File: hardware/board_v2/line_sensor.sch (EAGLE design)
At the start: 64 parts, among them J1 XF2L-0535-1, Q1 BSS123

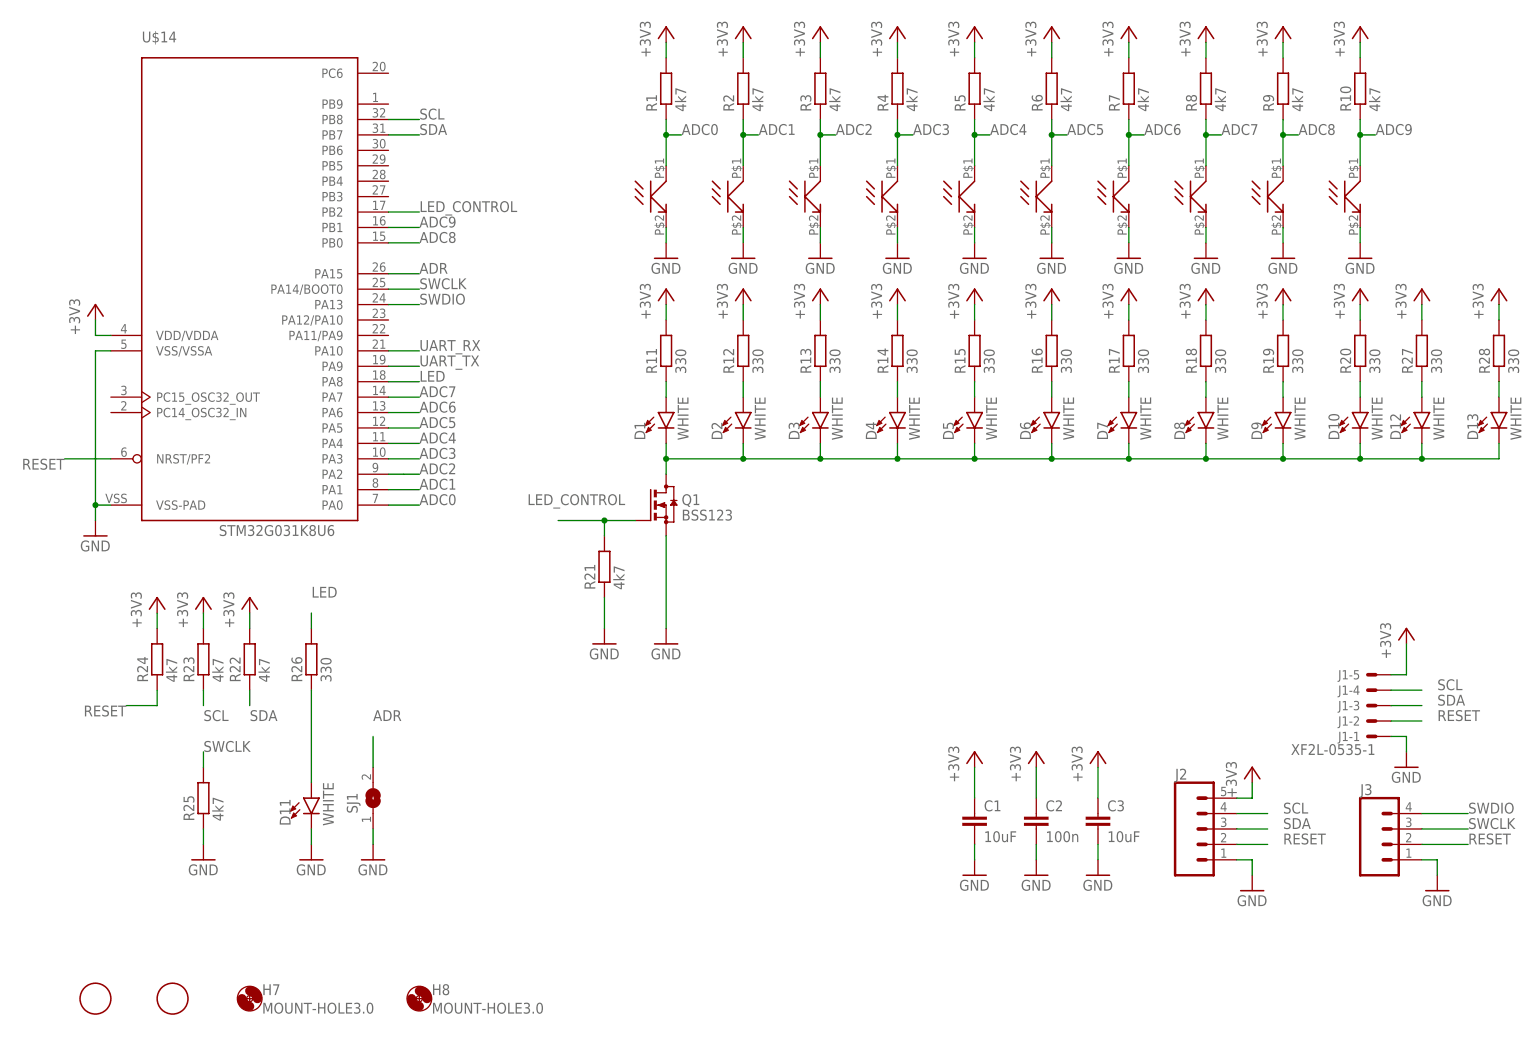
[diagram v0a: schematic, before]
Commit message: updated v2 firmware
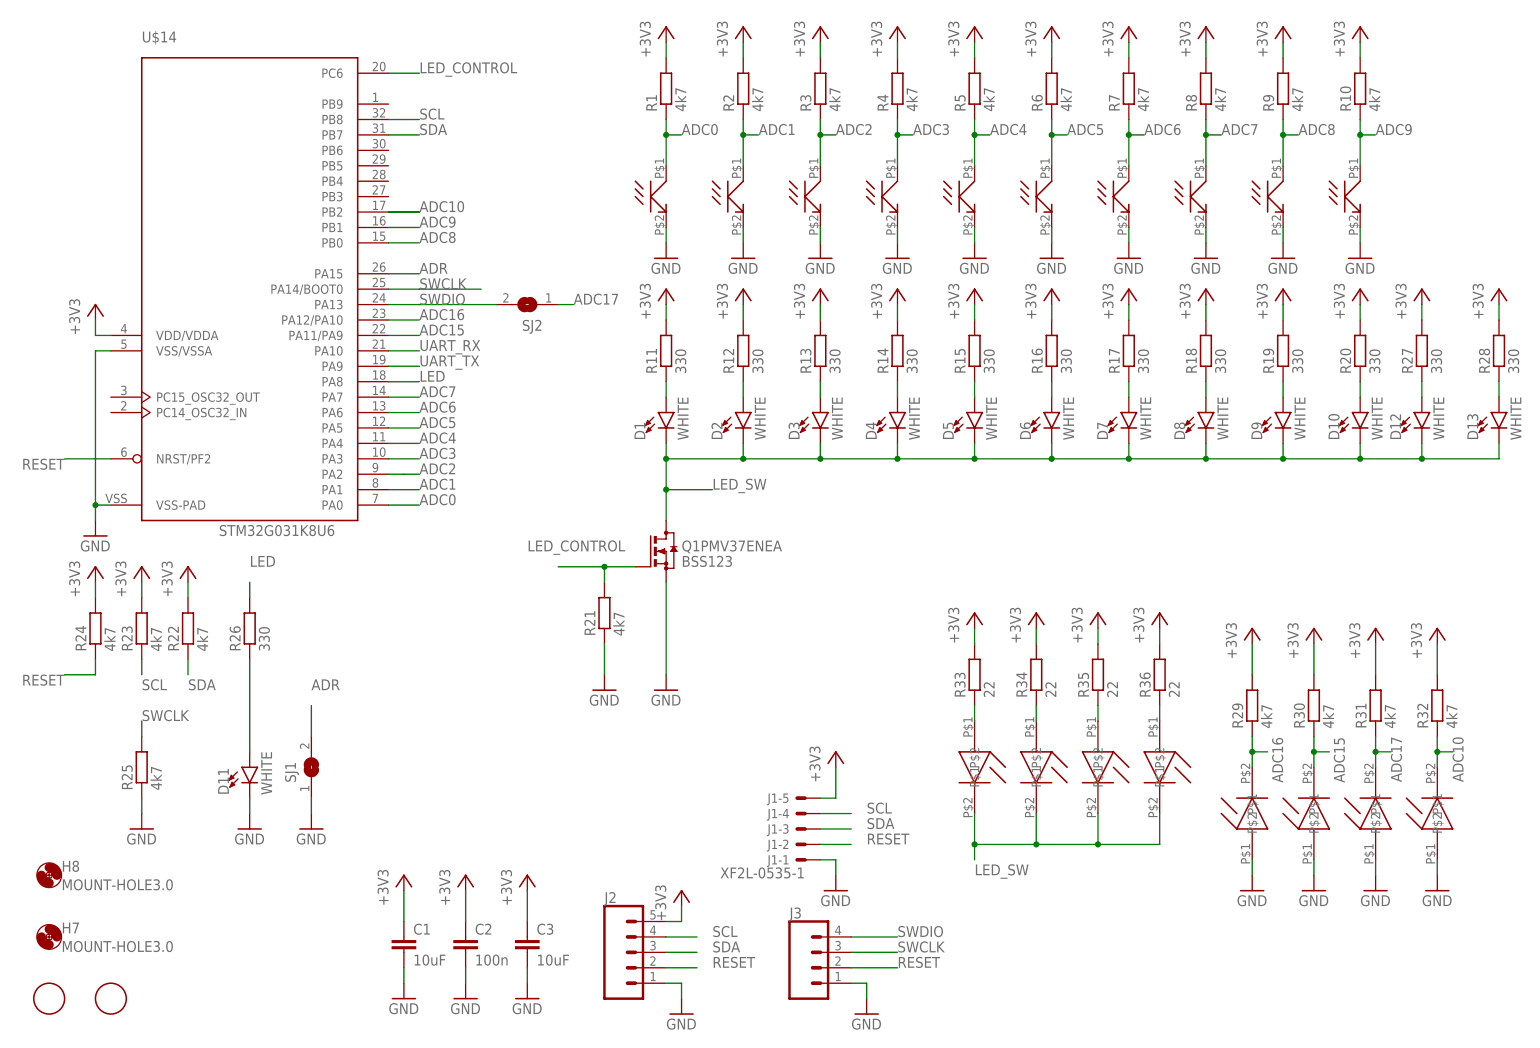
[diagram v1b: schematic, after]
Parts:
- removed Q1: BSS123, transistor-small-signal:BSS123
- added Q1PMV37ENEA: BSS123, transistor-small-signal:BSS123
- added R29, R30, R31, R32: 4k7, rcl:R-EU_M0805
- added R33, R34, R35, R36: 22, rcl:R-EU_M0805
- added SJ2: (no value), jumper:SJ
- added U$11, U$15, U$16, U$17, U$18, U$19, U$20, U$21: LED_5MM_AXIAL, my_library:LED_5MM_AXIAL
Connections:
- new net ADC10: R32.1, U$14.PB2, U$21.P$2
- new net ADC15: R30.1, U$14.PA11/PA9, U$17.P$2
- new net ADC16: R29.1, U$14.PA12/PA10, U$15.P$2
- new net ADC17: R31.1, SJ2.1, U$19.P$2
- new net LED_SW: D1.C, D10.C, D12.C, D13.C, D2.C, D3.C, D4.C, D5.C, D6.C, D7.C, D8.C, D9.C, Q1PMV37ENEA.D, U$11.P$2, U$16.P$2, U$18.P$2, U$20.P$2
- new net N$19: R34.1, U$16.P$1
- new net N$20: R35.1, U$18.P$1
- new net N$21: R36.1, U$20.P$1
- net +3V3: now also R29.2, R30.2, R31.2, R32.2, R33.2, R34.2, R35.2, R36.2
- net GND: now also Q1PMV37ENEA.S, U$15.P$1, U$17.P$1, U$19.P$1, U$21.P$1; no longer Q1.S
- net LED_CONTROL: now also Q1PMV37ENEA.G, U$14.PC6; no longer Q1.G, U$14.PB2
- net N$11: now also R33.1, U$11.P$1; no longer D1.C, D10.C, D12.C, D13.C, D2.C, D3.C, D4.C, D5.C, D6.C, D7.C, D8.C, D9.C, Q1.D
- net SWDIO: now also SJ2.2
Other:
- moved on the sheet: C1, C2, C3, D11, H7, H8, J1-1, J1-2, J1-3, J1-4, J1-5, J2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
